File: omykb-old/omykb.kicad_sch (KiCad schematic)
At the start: 183 parts, among them J2 USB_C_Receptacle_USB2.0_16P, K0 Esc, K1 !,1, K10 ),0, K11 _,-, K12 +,=, K13 Backspace, K14 Home, K15 Tab, K16 Q, K17 W, K18 E, K19 R, K2 @,2, K20 T, K21 Y, K22 U, K23 I, K24 O, K25 P, K26 {,[, K27 },], K28 |,\, K29 PgUp, K3 #,3, K30 Caps Lock, K31 A, K32 S, K33 D, K34 F, K35 G, K36 H, K37 J, K38 K, K39 L, K4 $,4, K40 :,;, K41 ",', K42 Enter, K43 PgDn, K44 Shift, K45 Z, K46 X, K47 C, K48 V, K49 B, K5 %,5, K50 N, K51 M, K52 <,,, K53 >,., K54 ?,/, K55 Shift, K56 ↑, K57 End, K58 Ctrl, K59 Cmd, K6 ^,6, K60 Alt, K61 Blank, K62 Alt, K63 Ctrl, K64 ←, K65 ↓, K66 →, K7 &,7, K8 *,8, K9 (,9, SW1 SW_Push, SW2 SW_Push, U1 RP2040, U2 NCP1117-3.3_SOT223, U4 W25Q128JVS, Y1 Crystal_GND24

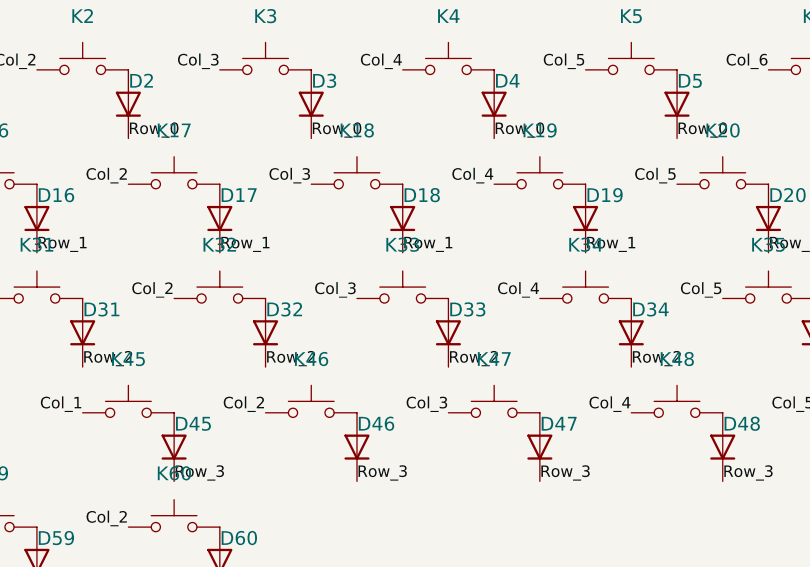
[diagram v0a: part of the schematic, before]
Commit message: trying again
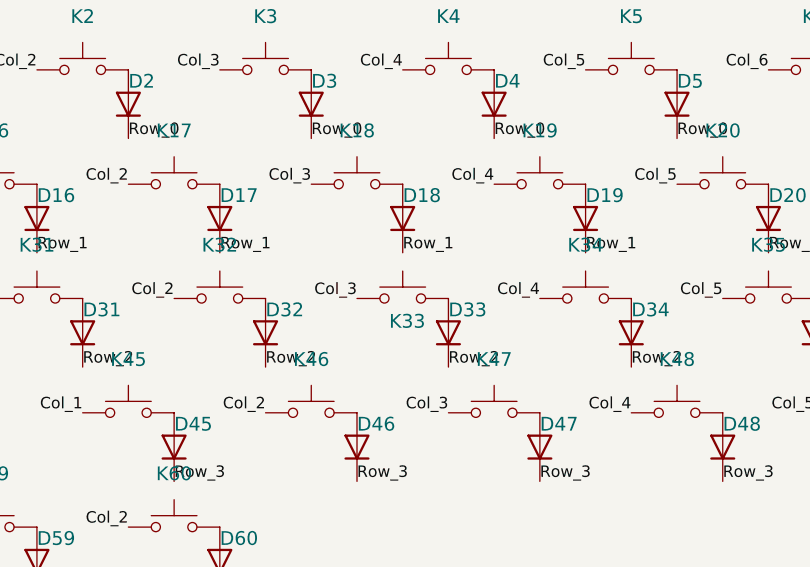
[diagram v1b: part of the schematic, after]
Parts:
- D0, D1, D10, D11, D12, D13, D14, D15, D16, D17, D18, D19, D2, D20, D21, D22, D23, D24, D25, D26, D27, D28, D29, D3, D30, D31, D32, D33, D34, D35, D36, D37, D38, D39, D4, D40, D41, D42, D43, D44, D45, D46, D47, D48, D49, D5, D50, D51, D52, D53, D54, D55, D56, D57, D58, D59, D6, D60, D61, D62, D63, D64, D65, D66, D7, D8, D9: value D -> 1N4148WS; footprint Diode_SMD:D_0805_2012Metric_Pad1.15x1.40mm_HandSolder -> Diode_SMD:D_SOD-323_HandSoldering
- K33: value D -> Key_D
